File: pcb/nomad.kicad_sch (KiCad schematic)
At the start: 35 parts, among them J1 USB_C_Receptacle_USB2.0_16P, SW1 UP, SW2 DOWN, SW3 RIGHT, SW4 LEFT, SW5 SEL, SW6 SW_Push, SW7 SW_Push, U1 ESP32-S3-WROOM-1, U2 PCF8574T, U3 MAX17048G_T10, U5 CH343G, U7 AMS1117-3.3

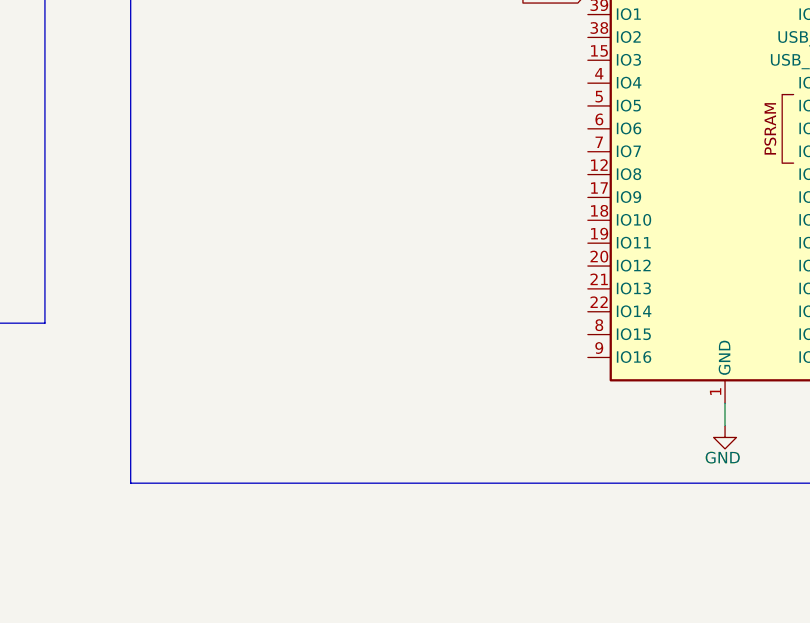
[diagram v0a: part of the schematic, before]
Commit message: Updating PCB
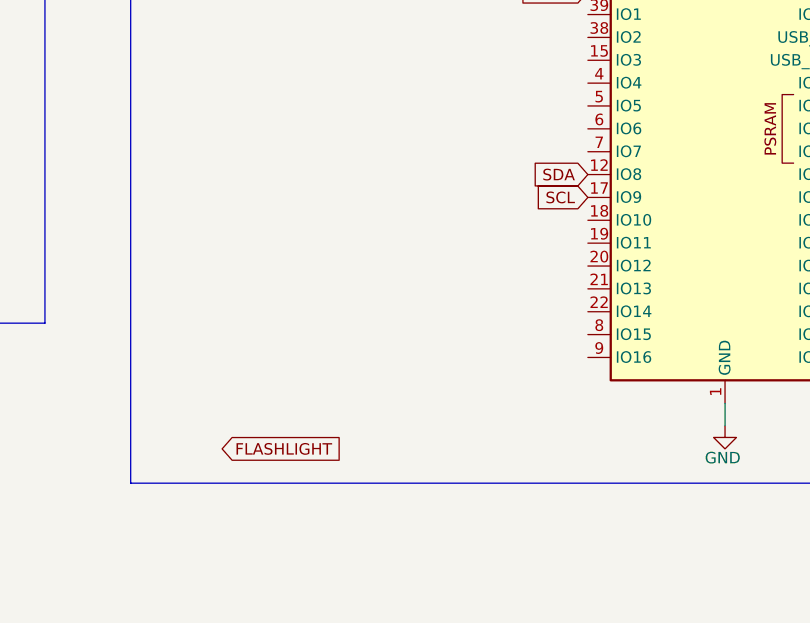
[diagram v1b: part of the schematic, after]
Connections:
- net SCL: now also U1.17 (IO9)
- net SDA: now also U1.12 (IO8)
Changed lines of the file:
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@@
+		)
+	)
+	(global_label "FLASHLIGHT"
+		(shape input)
+		(at 195.58 87.63 0)
+		(fields_autoplaced yes)
+		(effects
+			(font
+				(size 1.27 1.27)
+			)
+			(justify left)
+		)
+		(property "Intersheetrefs" "${INTERSHEET_REFS}"
+			(at 209.5115 87.63 0)
+			(hide yes)
+			(show_name no)
+			(do_not_autoplace no)
+			(effects
+				(font
+					(size 1.27 1.27)
+				)
+				(justify left)
+			)
 		)
 	)
@@
 		)
 	)
+	(global_label "SCL"
+		(shape input)
+		(at 236.22 59.69 180)
+		(fields_autoplaced yes)
+		(effects
+			(font
+				(size 1.27 1.27)
+			)
+			(justify right)
+		)
+		(property "Intersheetrefs" "${INTERSHEET_REFS}"
+			(at 229.7272 59.69 0)
+			(hide yes)
+			(show_name no)
+			(do_not_autoplace no)
+			(effects
+				(font
+					(size 1.27 1.27)
+				)
+				(justify right)
+			)
+		)
+	)
 	(global_label "BUTTON_INT"
 		(shape input)
@@
 			)
 		)
+	)
+	(global_label "SDA"
+		(shape input)
+		(at 236.22 57.15 180)
+		(fields_autoplaced yes)
+		(effects
+			(font
+				(size 1.27 1.27)
+			)
+			(justify right)
+		)
+		(property "Intersheetrefs" "${INTERSHEET_REFS}"
+			(at 229.6667 57.15 0)
+			(hide yes)
+			(show_name no)
+			(do_not_autoplace no)
+			(effects
+				(font
+					(size 1.27 1.27)
+				)
+				(justify right)
+			)
+		)
